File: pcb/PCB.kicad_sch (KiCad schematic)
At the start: 11 parts

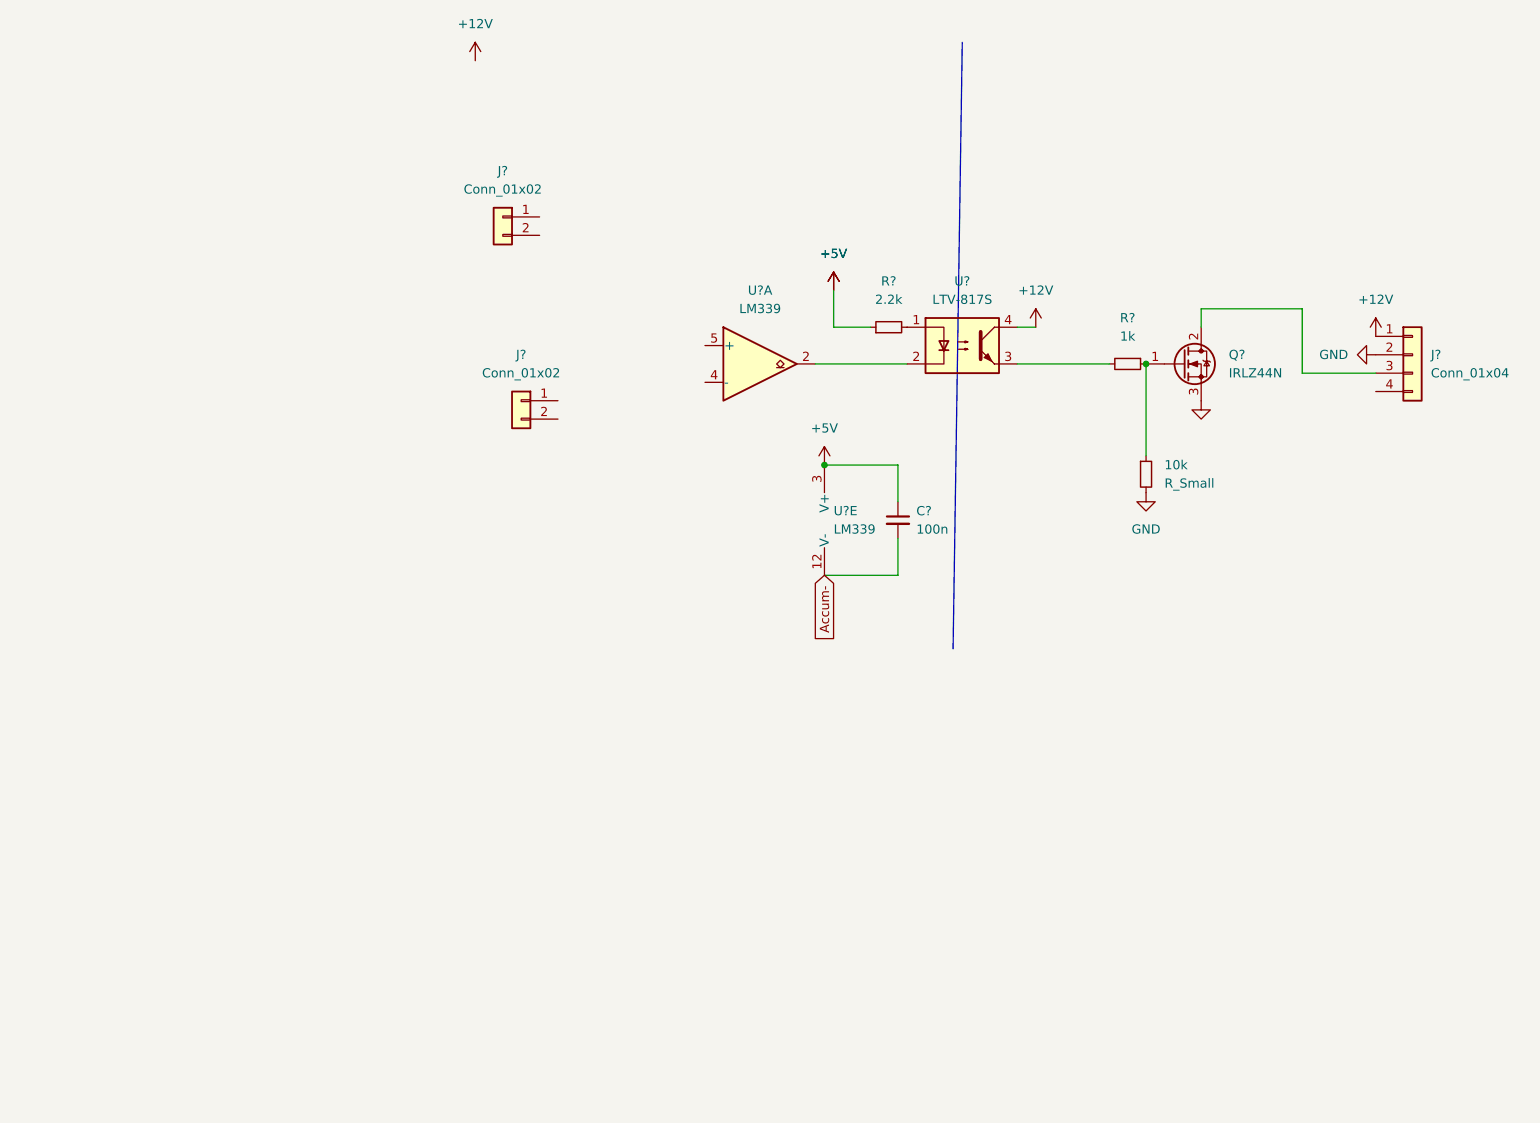
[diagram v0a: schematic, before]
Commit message: Precharge PCB update
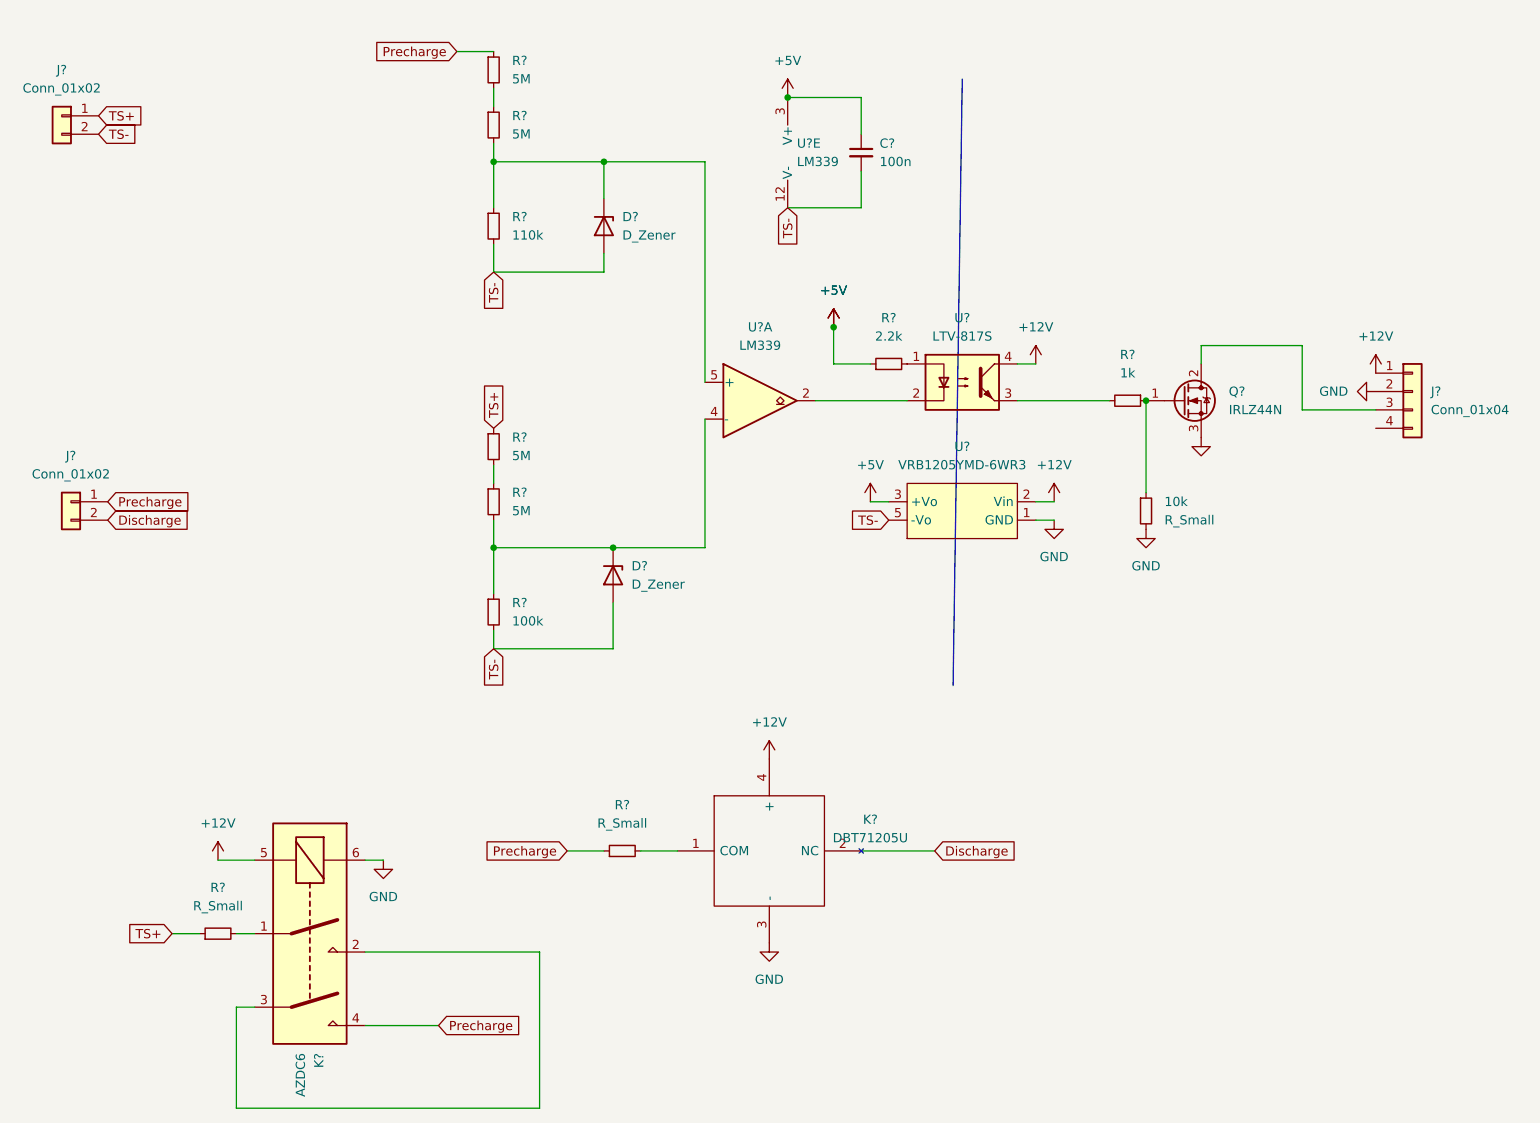
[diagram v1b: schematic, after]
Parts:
- added D? (x2): D_Zener, symbol Device:D_Zener
- added K?: DBT71205U, DBT71205U, symbol DBT71205U:DBT71205U
- added K?: AZDC6, symbol AZDC6:AZDC6
- added R? (x2): R_Small, symbol Device:R_Small
- added R?: 100k, symbol Device:R_Small
- added R? (x4): 5M, symbol Device:R_Small
- added R?: 110k, symbol Device:R_Small
- added U?: VRB1205YMD-6WR3, symbol VRB1205YMD-6WR3:VRB1205YMD-6WR3
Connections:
- net Accum- is gone; now on net TS-: C?.2, U?.12 (V-)
- net +12V: now also K?.4 (+), K?.5, U?.2 (Vin)
- net +5V: now also U?.3 (+Vo)
- net GND: now also K?.3 (-), K?.6, U?.1 (GND)
- net TS+: now reaches J?.1 (Pin_1)
- net TS+: now also R?.1, R?.1
- net TS-: now reaches J?.2 (Pin_2)
- net TS-: now also D?.2 (A), D?.2 (A), R?.2, R?.2, U?.5 (-Vo)
- net Precharge: now reaches J?.1 (Pin_1)
- net Precharge: now also K?.4, R?.1, R?.1
- net Discharge: now reaches J?.2 (Pin_2)
- net Discharge: now also K?.2 (NC)
- net at U?.4 (-): now also D?.1 (K), R?.1, R?.2
- net at U?.5 (+): now also D?.1 (K), R?.1, R?.2
- new net: K?.1 (COM), R?.2
- new net: K?.1, R?.2
- new net: R?.1, R?.2 (x2)
- new net: K?.2, K?.3
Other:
- moved on the sheet: 10k, C?, J?, Q?, R?, U?, U?A, U?E
